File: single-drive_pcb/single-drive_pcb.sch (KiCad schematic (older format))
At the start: 47 parts, among them IC1 MCP4232, IC2 ATMEGA328P_TQFP, IC3 DRV8834_SOP, IC4 MIC5205, IC5 BLE112-A, IC6 MAX1555, J1 MICROUSB, M1 STEPPER, P1 AVR_ISP, P2 CC_ISP, Y1 8MHz

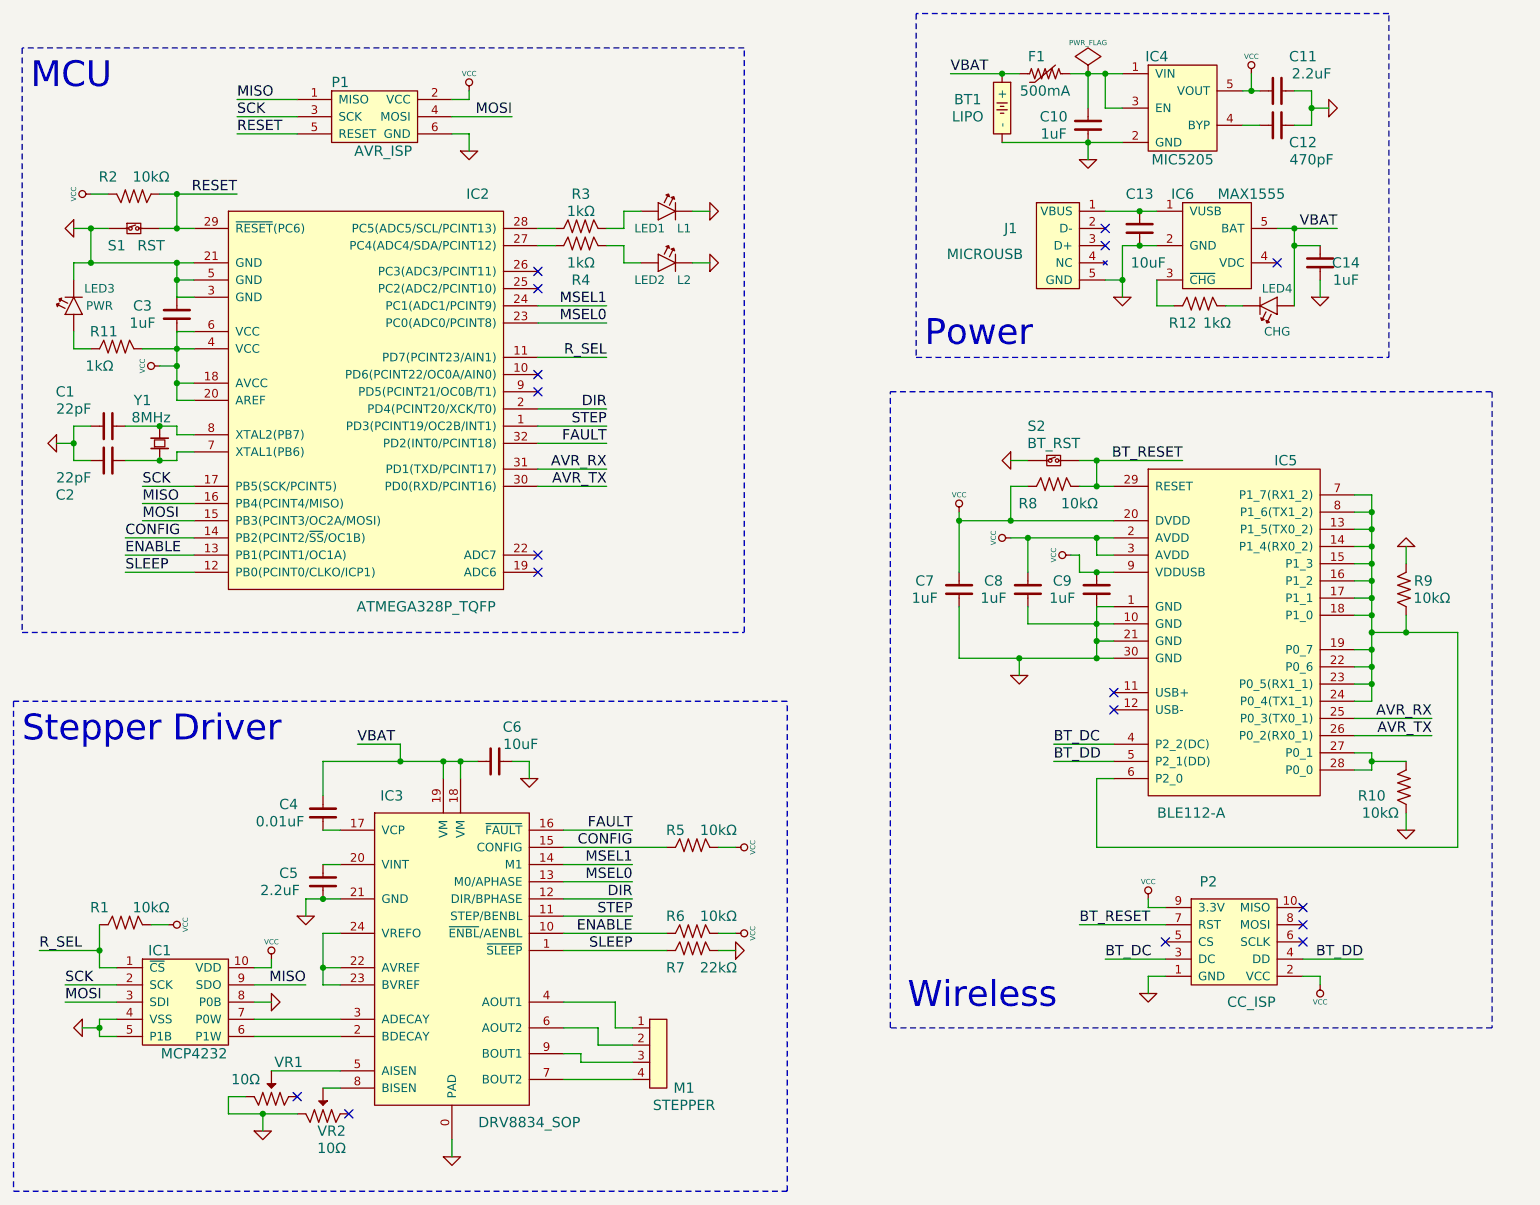
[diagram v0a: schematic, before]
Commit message: schematic done and footprints assigned
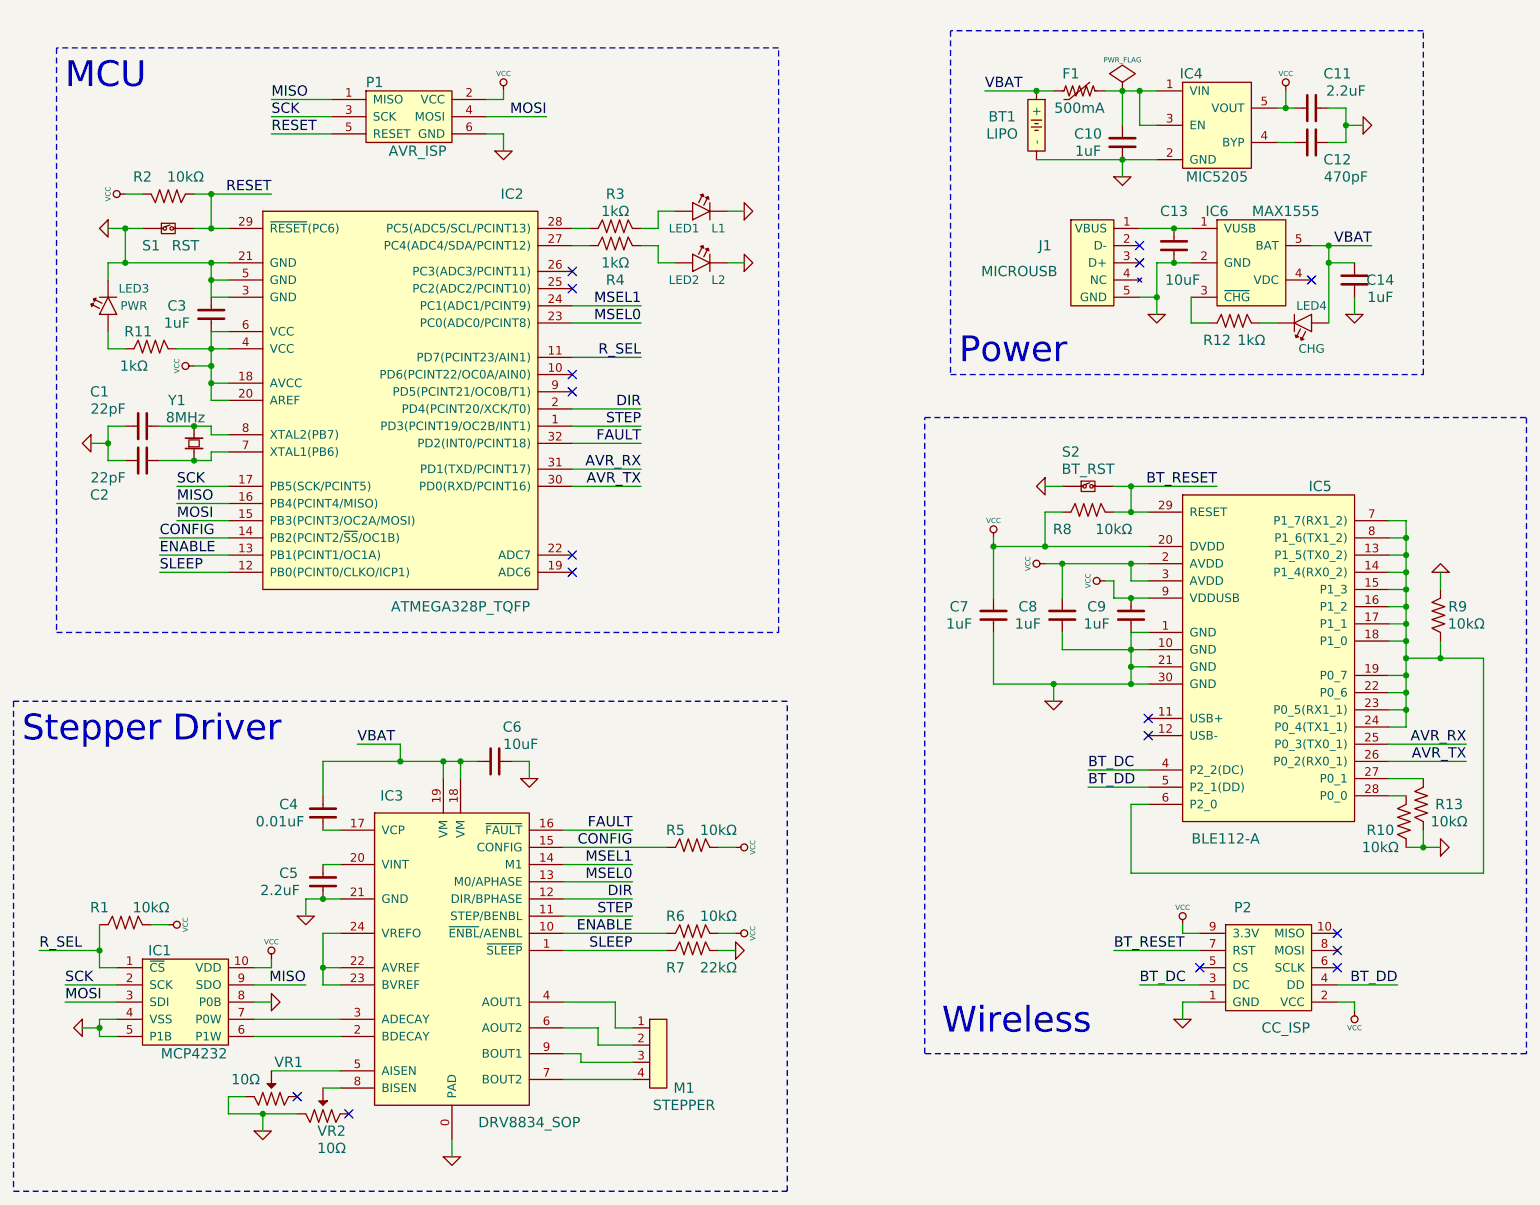
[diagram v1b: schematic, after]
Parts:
- added R13: 10kΩ, ~, symbol R
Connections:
- net GND: now also R13.1
- net at IC5.28 (P0_0), R10.2: no longer IC5.27 (P0_1)
- new net: IC5.27 (P0_1), R13.2
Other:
- moved on the sheet: BT1, C1, C10, C11, C12, C13, C14, C2, C3, C7, C8, C9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
